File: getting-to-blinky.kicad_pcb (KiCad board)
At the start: 2 copper layers, 30 x 22.8 mm, 11 parts, among them SW1 JS202011SCQN, U1 ICM7555

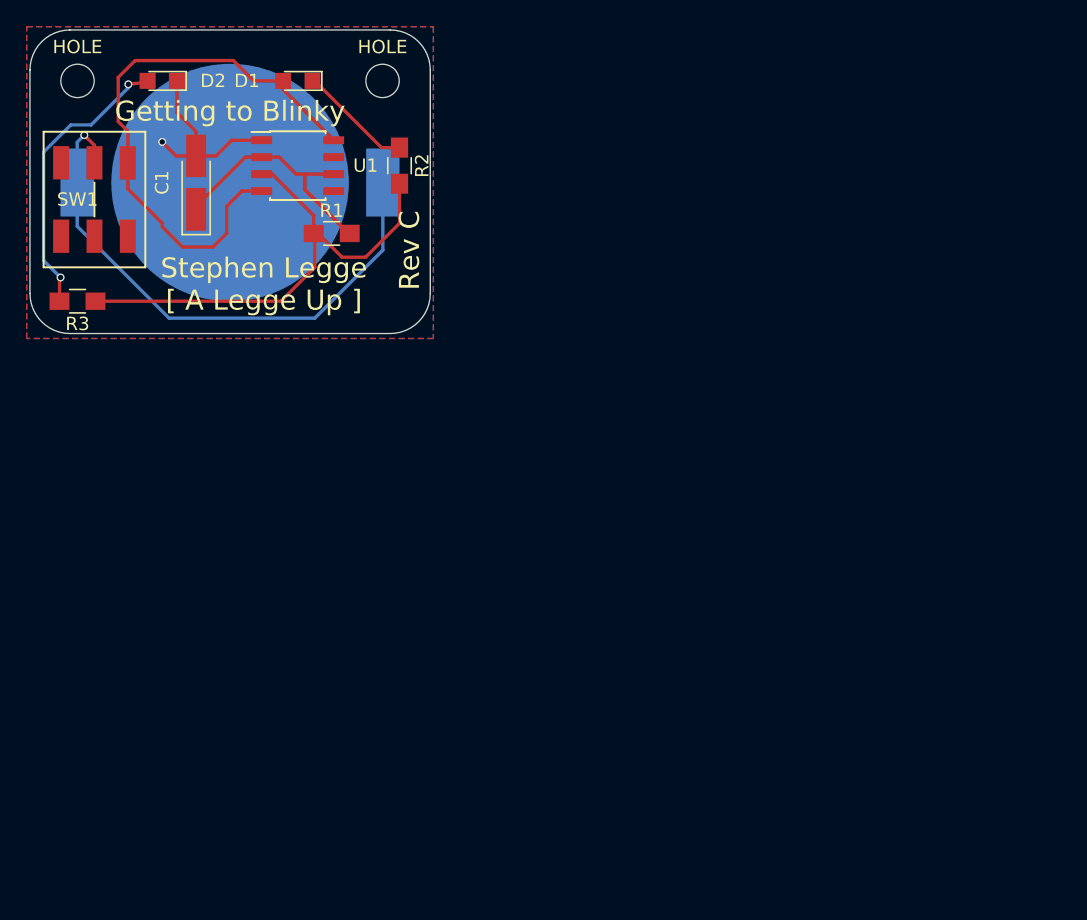
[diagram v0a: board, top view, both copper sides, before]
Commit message: Finalized and cleaned up the schematic and layed out Rev C
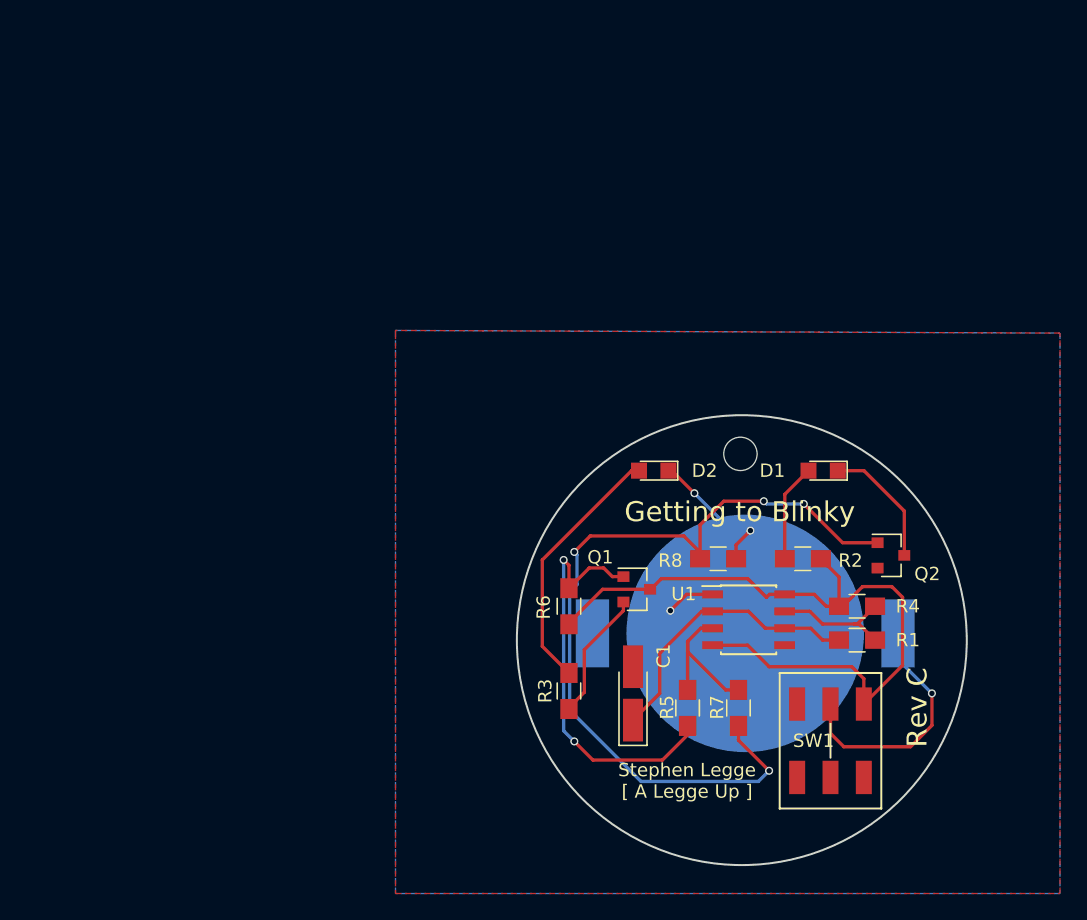
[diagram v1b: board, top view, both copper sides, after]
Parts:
- removed the HOLE at (160.0, 92.7)
- added Q1: BC808-40, TO_SOT_Packages_SMD:SOT-23, F.Cu at (179.1, 130.8)
- added Q2: BC818-40, TO_SOT_Packages_SMD:SOT-23, F.Cu at (198.1, 128.3)
- added R4: 470, Resistors_SMD:R_0805_HandSoldering, F.Cu at (195.6, 132.1)
- added R5: 1.2K, Resistors_SMD:R_0805_HandSoldering, F.Cu at (182.9, 139.7)
- added R6: 720, Resistors_SMD:R_0805_HandSoldering, F.Cu at (174.0, 132.1)
- added R7: 1.2K, Resistors_SMD:R_0805_HandSoldering, F.Cu at (186.7, 139.7)
- added R8: 720, Resistors_SMD:R_0805_HandSoldering, F.Cu at (185.2, 128.5)
- R1: value R -> 110K
- R2, R3: value R -> 55
- moved SW1 68.5 mm to (193.6, 142.2)
- moved HOLE 57.0 mm to (186.8, 120.7)
- moved BT1 51.3 mm to (187.2, 134.1)
- moved C1 50.4 mm to (178.8, 138.6)
- moved R1 49.8 mm to (195.6, 134.6), turned to 180 degrees
- moved D1 49.0 mm to (193.0, 121.9)
- moved U1 48.0 mm to (187.5, 133.1)
- moved D2 47.0 mm to (180.3, 121.9)
- moved R3 47.0 mm to (174.0, 138.4), turned to 270 degrees
- moved R2 42.2 mm to (191.5, 128.5), turned to 0 degrees
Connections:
- D1 pad 2: VCC -> Net-(D1-Pad2)
- R2 pad 1: Net-(D1-Pad1) -> Net-(D1-Pad2)
- R2 pad 2: Net-(R1-Pad1) -> VCC
- R3 pad 1: Net-(R1-Pad1) -> Net-(D2-Pad2)
- R3 pad 2: Net-(D2-Pad2) -> Net-(Q1-Pad2)
- U1 pad 3: Net-(R1-Pad1) -> /OUT
- U1 pad 7: (no net) -> Net-(R1-Pad1)
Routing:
- net Net-(Q2-Pad1): track 0.00 -> 62.8 mm, vias 0 -> 4
- net Net-(Q1-Pad1): track 0.00 -> 31.7 mm, vias 0 -> 2
- net Net-(R1-Pad1): track 37.8 -> 9.76 mm
- net Net-(BT1-Pad1): track 45.6 -> 18.8 mm
- net VCC: track 43.1 -> 56.1 mm
- net /OUT: track 0.00 -> 11.6 mm
- net Net-(Q1-Pad2): track 0.00 -> 9.71 mm
- net Net-(D1-Pad2): track 0.00 -> 7.34 mm
- net GND: track 29.4 -> 35.1 mm, vias 1 -> 3
- net Drain: track 25.0 -> 21.5 mm
- net Net-(D2-Pad2): track 21.9 -> 19.3 mm, vias 2 -> 0
- net Net-(D1-Pad1): track 8.59 -> 9.56 mm
- added copper zone on F.Cu, net GND
- added copper zone on B.Cu, net Net-(BT1-Pad1)
- removed copper zone on B.Cu, net GND
- removed copper zone on F.Cu, net VCC
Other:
- board size 30 x 22.8 mm -> 33.7 x 33.7 mm
